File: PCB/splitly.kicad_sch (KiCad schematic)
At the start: 122 parts, among them SW1 SW_Push_45deg, SW10 SW_Push_45deg, SW11 SW_Push_45deg, SW12 SW_Push_45deg, SW13 SW_Push_45deg, SW14 SW_Push_45deg, SW15 SW_Push_45deg, SW16 SW_Push_45deg, SW17 SW_Push_45deg, SW18 SW_Push_45deg, SW19 SW_Push_45deg, SW2 SW_Push_45deg, SW20 SW_Push_45deg, SW21 SW_Push_45deg, SW22 SW_Push_45deg, SW23 SW_Push_45deg, SW24 SW_Push_45deg, SW25 SW_Push_45deg, SW26 SW_Push_45deg, SW27 SW_Push_45deg, SW28 SW_Push_45deg, SW29 SW_Push_45deg, SW3 SW_Push_45deg, SW30 SW_Push_45deg, SW31 SW_Push_45deg, SW32 SW_Push_45deg, SW33 SW_Push_45deg, SW34 SW_Push_45deg, SW35 SW_Push_45deg, SW36 SW_Push_45deg, SW37 SW_Push_45deg, SW38 SW_Push_45deg, SW39 SW_Push_45deg, SW4 SW_Push_45deg, SW40 SW_Push_45deg, SW41 SW_Push_45deg, SW42 SW_Push_45deg, SW43 SW_Push_45deg, SW44 SW_Push_45deg, SW45 SW_Push_45deg, SW46 SW_Push_45deg, SW47 SW_Push_45deg, SW48 SW_Push_45deg, SW49 SW_Push_45deg, SW5 SW_Push_45deg, SW50 SW_Push_45deg, SW51 SW_Push_45deg, SW52 SW_Push_45deg, SW53 SW_Push_45deg, SW54 SW_Push_45deg, SW55 SW_Push_45deg, SW56 SW_Push_45deg, SW57 SW_Push_45deg, SW58 SW_Push_45deg, SW59 SW_Push_45deg, SW6 SW_Push_45deg, SW60 SW_Push_45deg, SW7 SW_Push_45deg, SW8 SW_Push_45deg, SW9 SW_Push_45deg, U1 XIAO-nRF52840-DIP, U2 XIAO-nRF52840-DIP

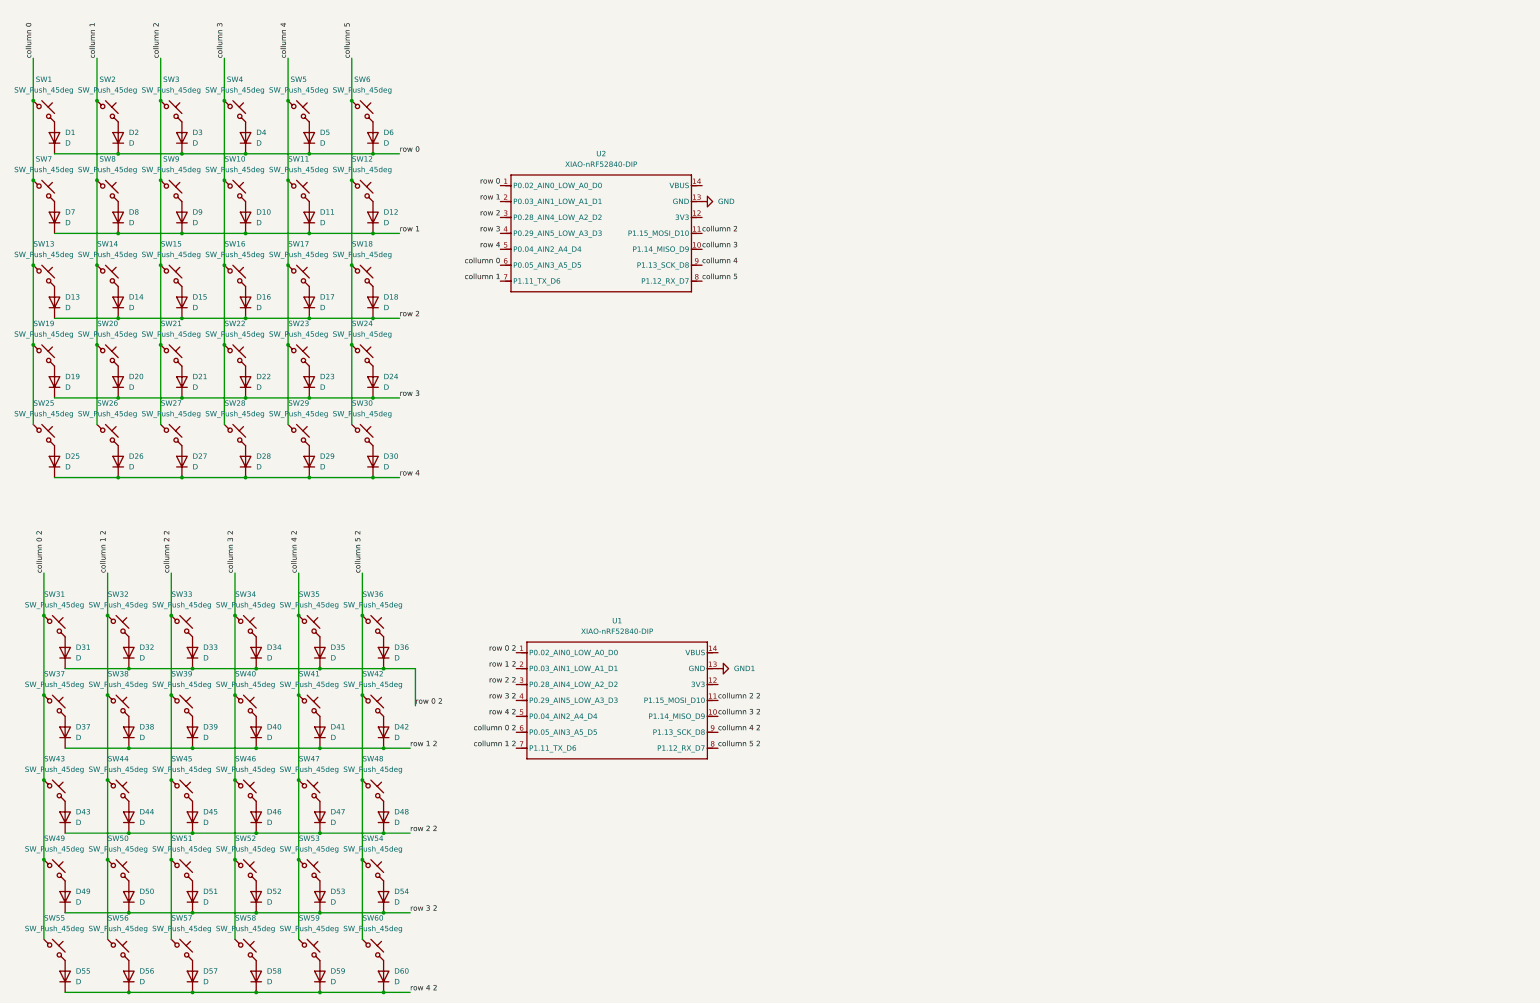
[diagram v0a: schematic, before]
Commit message: Add things to pcb
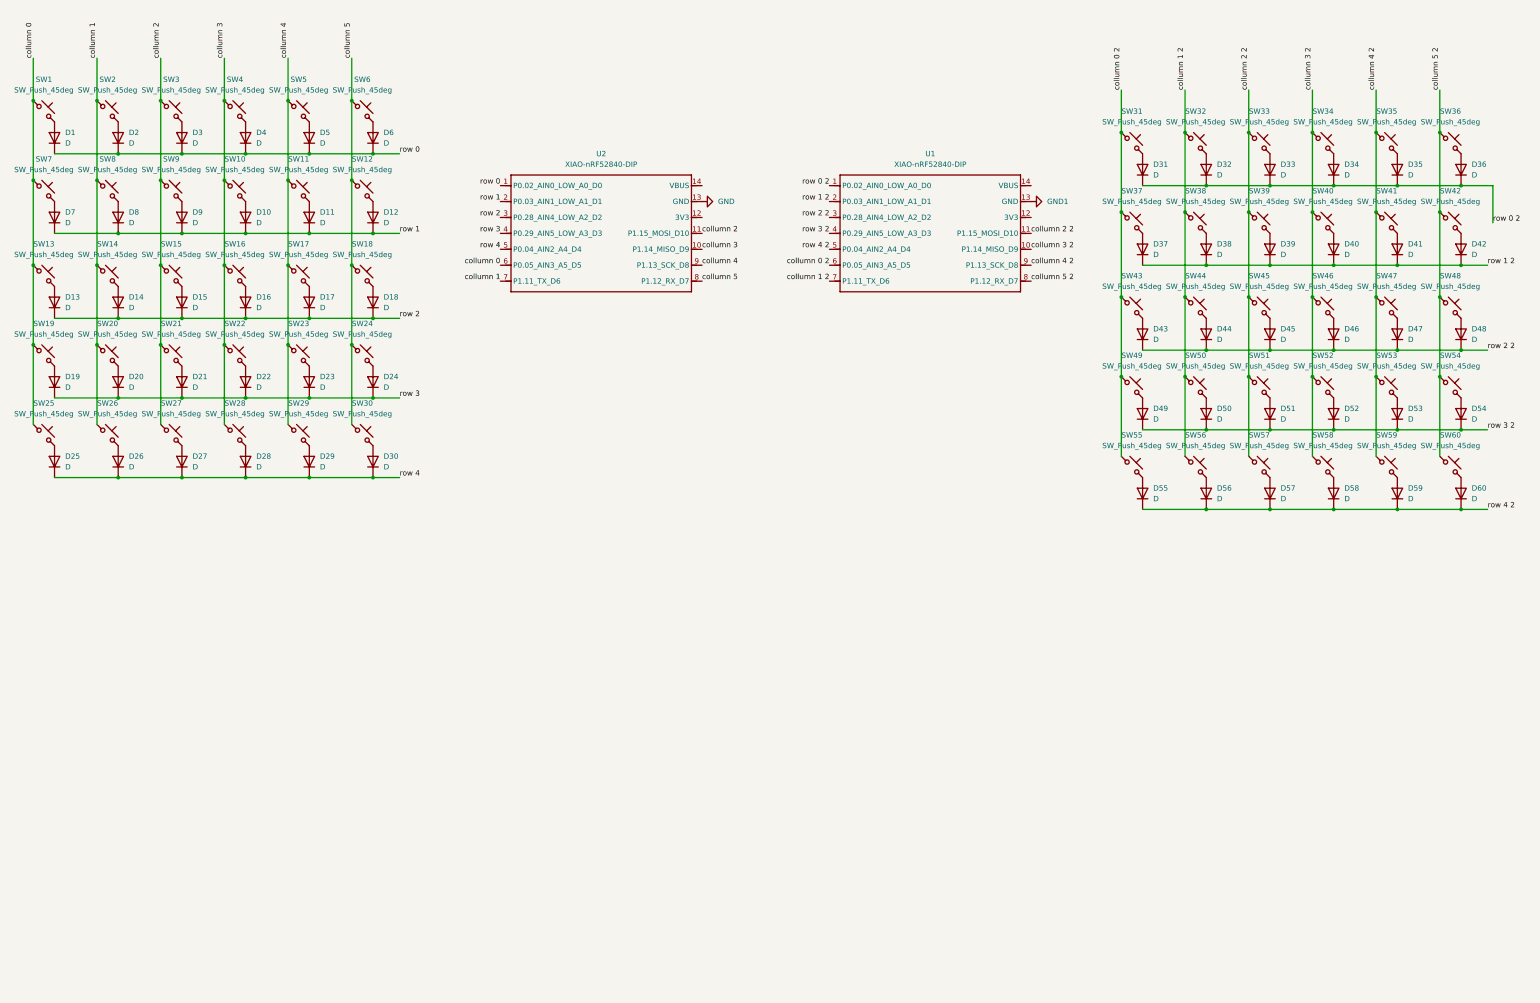
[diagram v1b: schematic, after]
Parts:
- D1, D10, D11, D12, D13, D14, D15, D16, D17, D18, D19, D2, D20, D21, D22, D23, D24, D25, D26, D27, D28, D29, D3, D30, D31, D32, D33, D34, D35, D36, D37, D38, D39, D4, D40, D41, D42, D43, D44, D45, D46, D47, D48, D49, D5, D50, D51, D52, D53, D54, D55, D56, D57, D58, D59, D6, D60, D7, D8, D9: footprint Diode_SMD:D_SOD-123 -> ScottoKeebs_Components:Diode_SOD-123
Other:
- moved on the sheet: D31, D32, D33, D34, D35, D36, D37, D38, D39, D40, D41, D42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
